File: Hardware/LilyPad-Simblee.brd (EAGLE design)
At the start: 45.3 x 45.2 mm, 37 parts, among them U1 MIC5219 3.3V, U2 MCP73831, U3 RFD77101

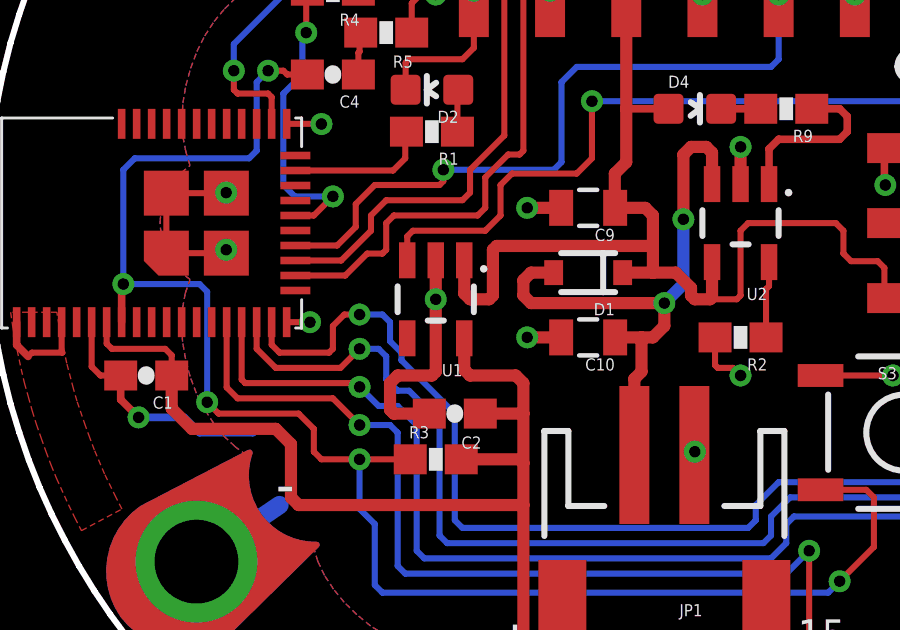
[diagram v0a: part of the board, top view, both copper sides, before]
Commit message: Release
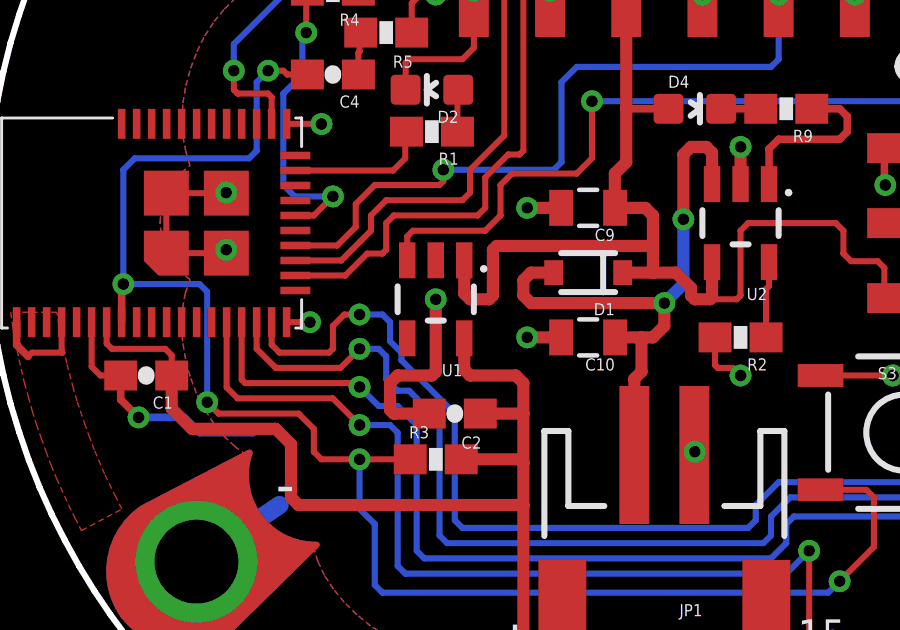
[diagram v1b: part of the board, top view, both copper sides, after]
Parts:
- U1: value MIC5219 3.3V -> ADP160
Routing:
- net GND: track 42.4 -> 41.1 mm
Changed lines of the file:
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@@
 <attribute name="PROD_ID" value="CAP-07888" x="-6.985" y="-6.35" size="1.778" layer="27" font="vector" ratio="15" rot="R180" display="off"/>
-</element>
-<element name="U1" library="SparkFun-PowerIC" package="SOT23-5" value="MIC5219 3.3V" x="-7.62" y="-2.54" rot="R180">
-<attribute name="PROD_ID" value="VREG-09872" x="-7.62" y="-2.54" size="1.778" layer="27" font="vector" ratio="15" rot="R180" display="off"/>
 </element>
 <element name="D1" library="SparkFun-DiscreteSemi" package="SOD-323" value="BAT20JFILM" x="-2.54" y="-1.651" rot="R180">
@@
 <element name="U$1" library="LilyPad-Wearables" package="LOGO-L" value="LOGO-LPL" x="9.144" y="6.096"/>
 <element name="U$2" library="LilyPad-Wearables" package="LOGO-LILYPAD" value="LOGO-LPLP" x="0.127" y="0.381" rot="MR0"/>
+<element name="U1" library="SparkFun-PowerIC" package="SOT23-5" value="ADP160" x="-7.62" y="-2.54" rot="R180">
+<attribute name="PROD_ID" value="VREG-11306" x="-7.62" y="-2.54" size="1.778" layer="27" font="vector" ratio="15" rot="R180" display="off"/>
+</element>
 </elements>
 <signals>
@@
 <contactref element="U3" pad="45"/>
 <contactref element="JP1" pad="1"/>
-<contactref element="U1" pad="2"/>
 <contactref element="S2" pad="3"/>
 <contactref element="C2" pad="2"/>
@@
 <wire x1="-3.44" y1="-3.81" x2="-4.572" y2="-3.81" width="0.4064" layer="1"/>
 <via x="-4.572" y="-3.81" extent="1-16" drill="0.381"/>
-<wire x1="-7.62" y1="-1.2399" x2="-7.62" y2="-2.54" width="0.4064" layer="1"/>
 <via x="-7.62" y="-2.54" extent="1-16" drill="0.381"/>
 <wire x1="2.54" y1="1.3001" x2="2.54" y2="2.54" width="0.4064" layer="1"/>
@@
 <wire x1="-15.494" y1="-6.985" x2="-13.716" y2="-6.985" width="0.254" layer="16"/>
 <wire x1="-13.716" y1="-6.985" x2="-13.589" y2="-6.858" width="0.254" layer="16"/>
+<contactref element="U1" pad="2"/>
 </signal>
 <signal name="RST">
@@
 <contactref element="U3" pad="7"/>
 <contactref element="C1" pad="1"/>
-<contactref element="U1" pad="5"/>
 <contactref element="C2" pad="1"/>
 <contactref element="U$43" pad="1"/>
@@
 <wire x1="-4.953" y1="-5.08" x2="-6.477" y2="-5.08" width="0.4064" layer="1"/>
 <wire x1="-6.477" y1="-5.08" x2="-6.67" y2="-4.887" width="0.4064" layer="1"/>
-<wire x1="-6.67" y1="-3.8401" x2="-6.67" y2="-4.887" width="0.4064" layer="1"/>
 <wire x1="-18.59" y1="-3.302" x2="-18.59" y2="-4.016" width="0.2032" layer="1"/>
 <wire x1="-18.59" y1="-4.016" x2="-18.415" y2="-4.191" width="0.2032" layer="1"/>
@@
 <wire x1="-15.748" y1="-6.858" x2="-12.954" y2="-6.858" width="0.4064" layer="1"/>
 <wire x1="-12.954" y1="-6.858" x2="-12.446" y2="-7.366" width="0.4064" layer="1"/>
+<contactref element="U1" pad="5"/>
+<wire x1="-6.67" y1="-4.887" x2="-6.67" y2="-3.8401" width="0.4064" layer="1"/>
 </signal>
 <signal name="N$1">
@@
 <contactref element="D4" pad="A"/>
 <contactref element="U2" pad="4"/>
-<contactref element="U1" pad="1"/>
 <contactref element="D1" pad="C"/>
 <contactref element="S2" pad="1"/>
@@
 <wire x1="7.112" y1="-1.27" x2="7.335" y2="-1.493" width="0.2032" layer="1"/>
 <wire x1="7.335" y1="-2.5" x2="7.335" y2="-1.493" width="0.2032" layer="1"/>
-<wire x1="-6.67" y1="-1.2399" x2="-6.67" y2="-2.347" width="0.4064" layer="1"/>
 <wire x1="-6.67" y1="-2.347" x2="-6.477" y2="-2.54" width="0.4064" layer="1"/>
 <wire x1="-6.477" y1="-2.54" x2="-5.842" y2="-2.54" width="0.4064" layer="1"/>
@@
 <wire x1="-5.715" y1="-2.413" x2="-5.715" y2="-0.889" width="0.4064" layer="1"/>
 <wire x1="-5.715" y1="-0.889" x2="-5.588" y2="-0.762" width="0.4064" layer="1"/>
+<contactref element="U1" pad="1"/>
+<wire x1="-6.67" y1="-1.2399" x2="-6.67" y2="-2.347" width="0.4064" layer="1"/>
 </signal>
 <signal name="V_BATT">
@@
 <signal name="N$3">
 <contactref element="S2" pad="2"/>
-<contactref element="U1" pad="3"/>
-<wire x1="-8.57" y1="-1.2399" x2="-8.57" y2="-0.442" width="0.2032" layer="1"/>
 <wire x1="-8.57" y1="-0.442" x2="-8.382" y2="-0.254" width="0.2032" layer="1"/>
 <wire x1="-8.382" y1="-0.254" x2="-5.969" y2="-0.254" width="0.2032" layer="1"/>
@@
 <via x="8.89" y="0" extent="1-16" drill="0.381"/>
 <wire x1="8.89" y1="0" x2="7.335" y2="0" width="0.2032" layer="1"/>
+<contactref element="U1" pad="3"/>
+<wire x1="-8.57" y1="-1.2399" x2="-8.57" y2="-0.442" width="0.2032" layer="1"/>
 </signal>
 <signal name="LV_RXI">
